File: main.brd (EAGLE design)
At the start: 24.4 x 26.2 mm, 46 parts, among them IC1 ATTINY13A-SSH, IC2 TP4056-42-ESOP8, IC3 LM27313XMFX_NOPB, IC4 TPL5110DDCT, IC5 ATTINY13A-SSH, T1A 2N4401, T1B NPN, X1 MINI-USB-UX60A-MB-5ST, X2 332-02

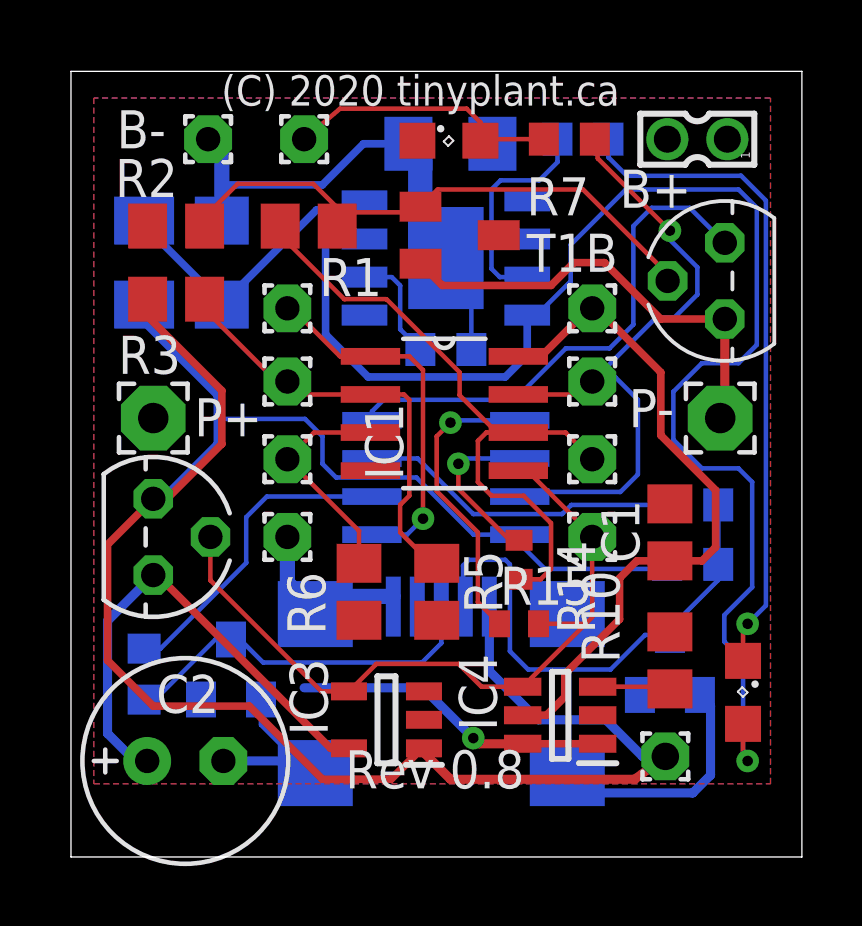
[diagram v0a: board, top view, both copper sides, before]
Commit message: lots of updates
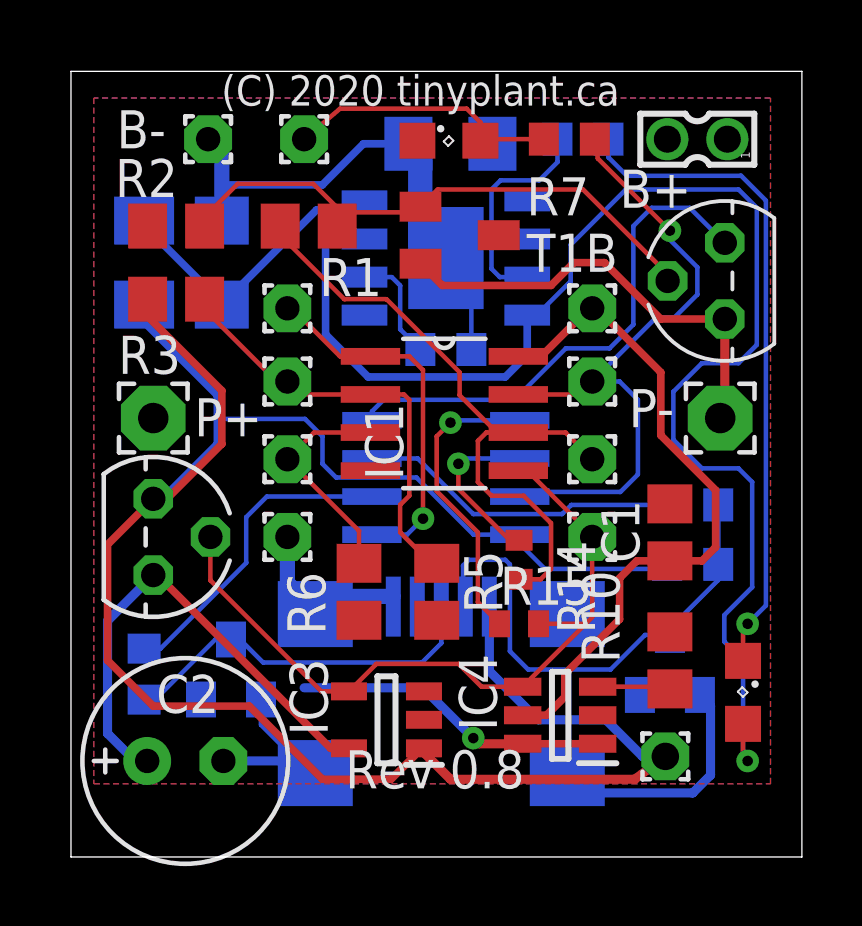
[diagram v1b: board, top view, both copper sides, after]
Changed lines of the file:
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@@
 <wire x1="17.8562" y1="14.5034" x2="15.8242" y2="14.5034" width="0.1524" layer="1"/>
 <contactref element="R7" pad="1"/>
-<wire x1="19.05" y1="15.0876" x2="18.4404" y2="15.0876" width="0.1524" layer="16"/>
-<wire x1="18.4404" y1="15.0876" x2="18.288" y2="14.9352" width="0.1524" layer="16"/>
+<wire x1="19.2024" y1="14.9352" x2="18.288" y2="14.9352" width="0.1524" layer="16"/>
 <wire x1="21.7932" y1="18.7452" x2="20.8788" y2="19.6596" width="0.1524" layer="16"/>
 <wire x1="20.8788" y1="19.9644" x2="20.8788" y2="19.6596" width="0.1524" layer="16"/>
@@
 <wire x1="19.2278" y1="11.2522" x2="19.812" y2="11.8364" width="0.1524" layer="16"/>
 <wire x1="19.812" y1="11.8364" x2="19.812" y2="14.3256" width="0.1524" layer="16"/>
-<wire x1="19.812" y1="14.3256" x2="19.05" y2="15.0876" width="0.1524" layer="16"/>
+<wire x1="19.812" y1="14.3256" x2="19.2024" y2="14.9352" width="0.1524" layer="16"/>
 <wire x1="21.7932" y1="17.8308" x2="21.0312" y2="17.0688" width="0.1524" layer="16"/>
 <wire x1="21.0312" y1="17.0688" x2="20.4216" y2="17.0688" width="0.1524" layer="16"/>

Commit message: rev 0.9
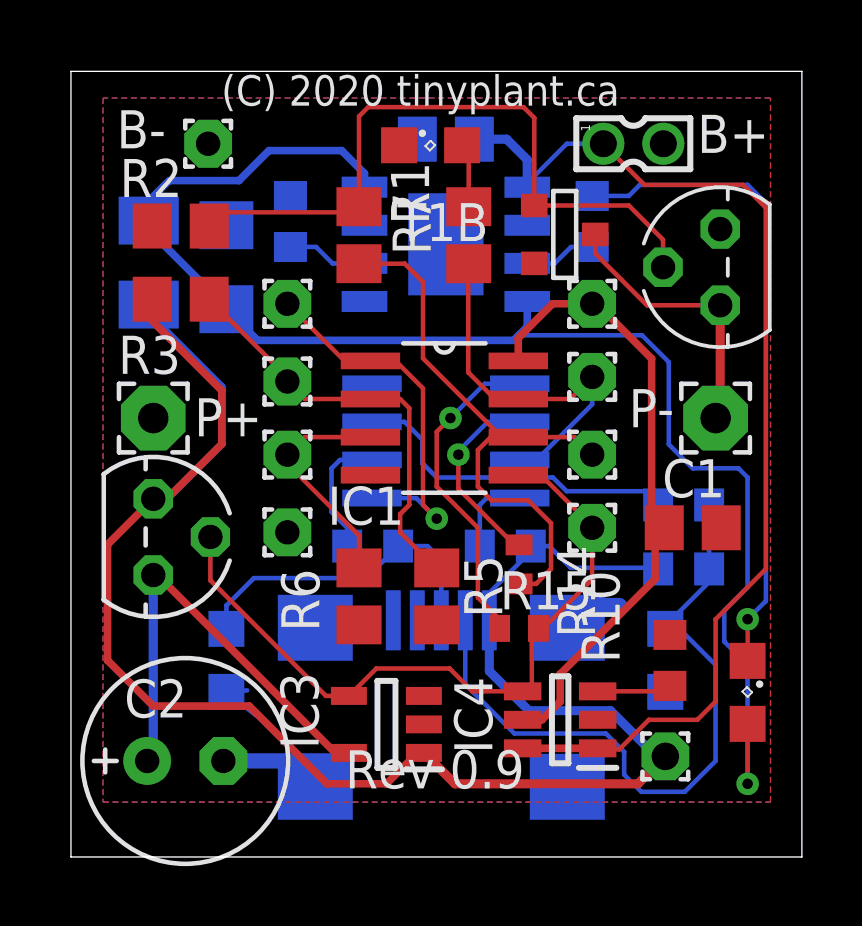
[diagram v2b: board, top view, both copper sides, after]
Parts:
- removed PAD1: (no value), wirepad:1,6/0,8
- added R16: 100R, resistor:R0603
- C4: device rcl:C1206 -> rcl:C0805
- D1, D2: value BZX84CSMD -> (none); device diode:TO236 -> led:SML0805
- R1: value 1k -> 100R
- R10: device resistor:R0805 -> resistor:R0603
- R13: value 1.5k -> 2.2k
- R7: device resistor:R0603 -> resistor:R0805
- T1B: device semicon-smd-ipc:SOT23W -> zetex:SOT-23
- moved R12 8.73 mm to (11.0, 9.45), turned to 0 degrees
- moved R9 6.71 mm to (8.23, 20.3), turned to 90 degrees
- moved R7 4.64 mm to (14.2, 19.8), turned to 90 degrees
- moved T1B 3.51 mm to (17.4, 19.8), turned to 90 degrees
- moved R8 2.76 mm to (18.3, 20.3), turned to 270 degrees
- moved X2 2.14 mm to (19.7, 22.9), turned to 270 degrees
- moved R1 1.70 mm to (10.5, 19.8), turned to 270 degrees
- moved IC5 1.22 mm to (13.4, 13.0)
- moved C1 0.78 mm to (21.6, 10.1), turned to 180 degrees
- moved LED1 0.63 mm to (12.9, 22.8)
- moved T1A 0.48 mm to (22.6, 18.7)
- moved IC2 0.46 mm to (13.4, 19.5)
- moved X1 0.46 mm to (13.3, 4.72)
- moved D2 0.34 mm to (6.10, 5.64), turned to 270 degrees
- moved R13 0.34 mm to (21.3, 8.69)
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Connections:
- new net N$17: IC5.8, R16.1
- net GND: now also T1B.2; no longer T1B.3
- net N$1: now also T1B.3; no longer T1B.1
- net N$2: now also T1B.1; no longer T1B.2
- net N$5: now also R16.2; no longer IC5.8
- net N$6: no longer PAD1.1
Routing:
- net GND: track 56.6 -> 9.33 mm
- net VCC: track 10.6 -> 36.7 mm, vias 1 -> 0
- net N$5: track 71.9 -> 61.4 mm
- net LED: track 22.4 -> 12.5 mm, vias 1 -> 0
- net N$4: track 57.6 -> 48.9 mm
- net N$6: track 9.18 -> 2.27 mm
- net N$12: track 10.6 -> 4.27 mm
- net N$13: track 17.1 -> 22.9 mm
- net N$2: track 14.9 -> 9.34 mm
- net N$8: track 7.29 -> 2.39 mm
- net N$1: track 19.0 -> 23.0 mm
- net N$17: track 0.00 -> 2.80 mm
- net NPN+: track 22.8 -> 20.4 mm
- net N$3: track 22.9 -> 21.0 mm
- net N$14: track 12.5 -> 11.0 mm
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- added copper zone on layer 16, net GND
- removed copper zone on layer 16, net VCC
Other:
- board text added: "Rev 0.9"
- board text removed: "Rev 0.8"
